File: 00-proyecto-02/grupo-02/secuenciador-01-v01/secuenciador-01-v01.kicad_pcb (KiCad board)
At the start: 2 copper layers, 90 x 50 mm, 18 parts, among them U1 4040, U2 NE555P

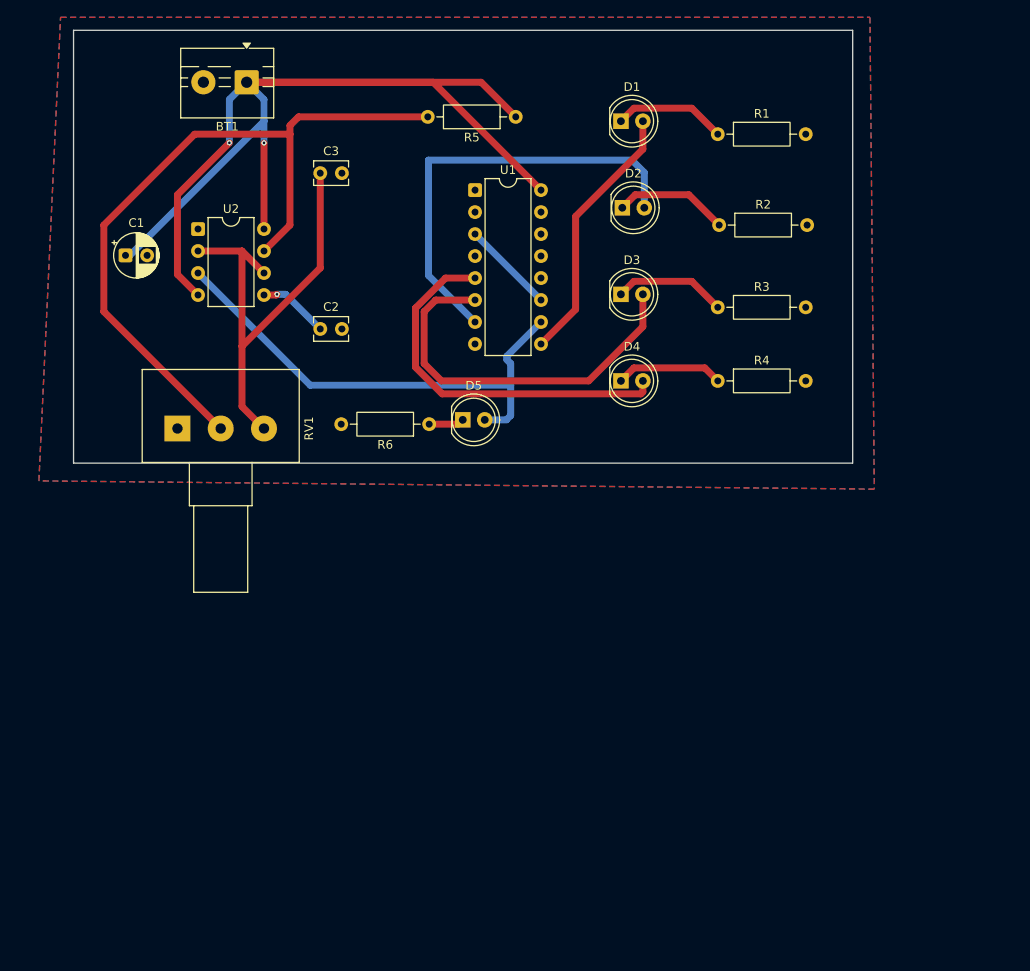
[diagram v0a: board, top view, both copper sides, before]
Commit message: Add files via upload
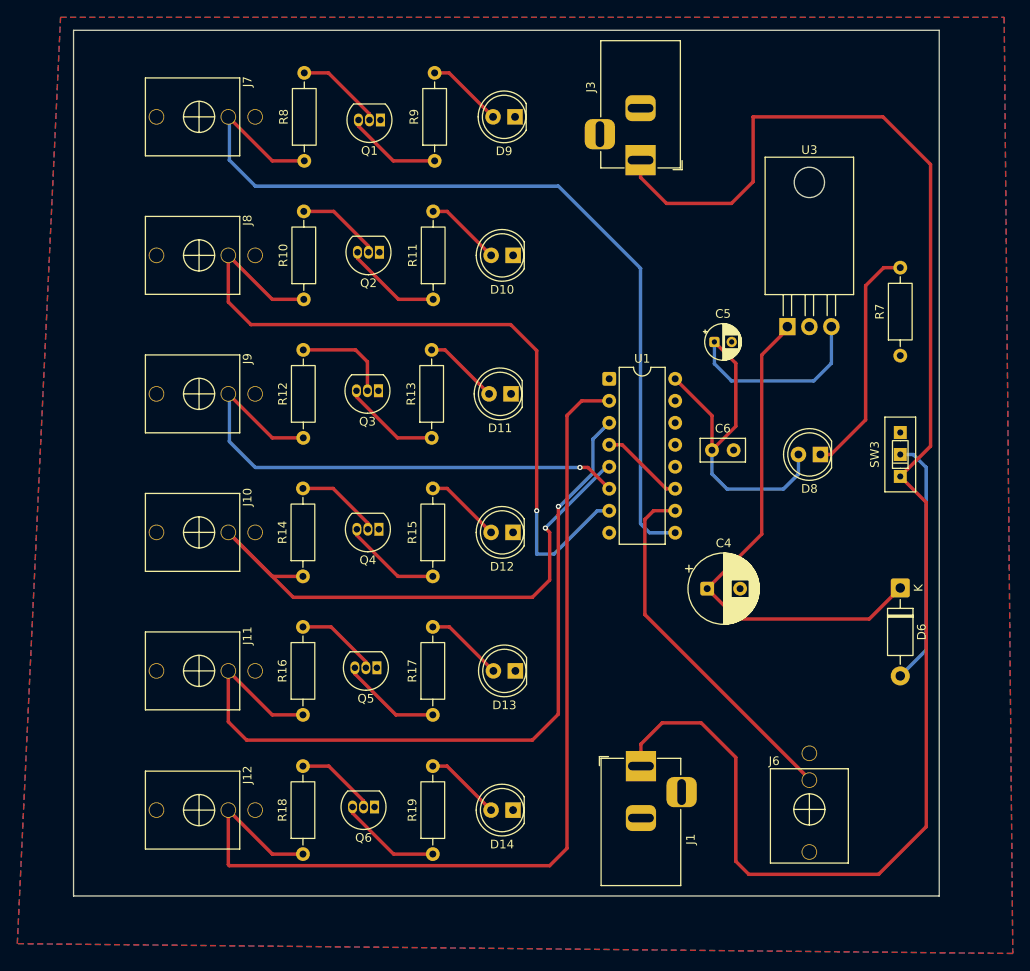
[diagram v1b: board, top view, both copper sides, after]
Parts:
- removed BT1: 9v, TerminalBlock:TerminalBlock_MaiXu_MX126-5.0-02P_1x02_P5.00mm
- removed C1: 100u, Capacitor_THT:CP_Radial_D5.0mm_P2.50mm
- removed C2: 100n, Capacitor_THT:C_Disc_D3.8mm_W2.6mm_P2.50mm
- removed C3: 10n, Capacitor_THT:C_Disc_D3.8mm_W2.6mm_P2.50mm
- removed D1, D2, D3, D4, D5: LED, LED_THT:LED_D5.0mm
- removed R1, R2, R3, R4, R6: 1k, Resistor_THT:R_Axial_DIN0207_L6.3mm_D2.5mm_P10.16mm_Horizontal
- removed R5: 10k, Resistor_THT:R_Axial_DIN0207_L6.3mm_D2.5mm_P10.16mm_Horizontal
- removed RV1: 100k, Potentiometer_THT:Potentiometer_Alps_RK163_Single_Horizontal
- removed U2: NE555P, Package_DIP:DIP-8_W7.62mm
- added C4: 100u, Capacitor_THT:CP_Radial_D8.0mm_P3.80mm, F.Cu at (123.7, 114.5)
- added C5: 10u, Capacitor_THT:CP_Radial_D4.0mm_P2.00mm, F.Cu at (124.5, 86.0)
- added C6: 100n, Capacitor_THT:C_Disc_D5.0mm_W2.5mm_P2.50mm, F.Cu at (124.2, 98.5)
- added D10: LED, LED_THT:LED_D5.0mm, F.Cu at (101.3, 76.0)
- added D11: LED, LED_THT:LED_D5.0mm, F.Cu at (101.0, 92.0)
- added D12: LED, LED_THT:LED_D5.0mm, F.Cu at (101.3, 108.0)
- added D13: LED, LED_THT:LED_D5.0mm, F.Cu at (101.5, 124.0)
- added D14: LED, LED_THT:LED_D5.0mm, F.Cu at (101.3, 140.1)
- added D6: 1N4007, Diode_THT:D_DO-41_SOD81_P10.16mm_Horizontal, F.Cu at (146.0, 114.4)
- added D8: LED, LED_THT:LED_D5.0mm, F.Cu at (136.8, 99.0)
- added D9: LED, LED_THT:LED_D5.0mm, F.Cu at (101.5, 60.0)
- added J1: Barrel_Jack_Switch, Connector_BarrelJack:BarrelJack_Horizontal, F.Cu at (116.0, 135.0)
- added J10: AudioJack2_SwitchT, dis8644:PJ301M-12, F.Cu at (65.0, 108.0)
- added J11: AudioJack2_SwitchT, dis8644:PJ301M-12, F.Cu at (65.0, 124.0)
- added J12: AudioJack2_SwitchT, dis8644:PJ301M-12, F.Cu at (65.0, 140.1)
- added J3: Barrel_Jack_Switch, Connector_BarrelJack:BarrelJack_Horizontal, F.Cu at (116.0, 65.0)
- added J6: AudioJack2_SwitchT, dis8644:PJ301M-12, F.Cu at (135.5, 140.0)
- added J7: AudioJack2_SwitchT, dis8644:PJ301M-12, F.Cu at (65.0, 60.0)
- added J8: AudioJack2_SwitchT, dis8644:PJ301M-12, F.Cu at (65.0, 76.0)
- added J9: AudioJack2_SwitchT, dis8644:PJ301M-12, F.Cu at (65.0, 92.0)
- added Q1: PN2222A, Package_TO_SOT_THT:TO-92_Inline, F.Cu at (86.0, 60.4)
- added Q2: PN2222A, Package_TO_SOT_THT:TO-92_Inline, F.Cu at (85.8, 75.6)
- added Q3: PN2222A, Package_TO_SOT_THT:TO-92_Inline, F.Cu at (85.7, 91.6)
- added Q4: PN2222A, Package_TO_SOT_THT:TO-92_Inline, F.Cu at (85.8, 107.6)
- added Q5: PN2222A, Package_TO_SOT_THT:TO-92_Inline, F.Cu at (85.5, 123.6)
- added Q6: PN2222A, Package_TO_SOT_THT:TO-92_Inline, F.Cu at (85.3, 139.7)
- added R10: 1k, Resistor_THT:R_Axial_DIN0207_L6.3mm_D2.5mm_P10.16mm_Horizontal, F.Cu at (77.1, 81.1)
- added R11: 1k, Resistor_THT:R_Axial_DIN0207_L6.3mm_D2.5mm_P10.16mm_Horizontal, F.Cu at (92.0, 81.1)
- added R12: 1k, Resistor_THT:R_Axial_DIN0207_L6.3mm_D2.5mm_P10.16mm_Horizontal, F.Cu at (77.0, 97.1)
- added R13: 1k, Resistor_THT:R_Axial_DIN0207_L6.3mm_D2.5mm_P10.16mm_Horizontal, F.Cu at (91.9, 97.1)
- added R14: 1k, Resistor_THT:R_Axial_DIN0207_L6.3mm_D2.5mm_P10.16mm_Horizontal, F.Cu at (77.0, 113.1)
- added R15: 1k, Resistor_THT:R_Axial_DIN0207_L6.3mm_D2.5mm_P10.16mm_Horizontal, F.Cu at (92.0, 113.1)
- added R16: 1k, Resistor_THT:R_Axial_DIN0207_L6.3mm_D2.5mm_P10.16mm_Horizontal, F.Cu at (77.0, 129.1)
- added R17: 1k, Resistor_THT:R_Axial_DIN0207_L6.3mm_D2.5mm_P10.16mm_Horizontal, F.Cu at (92.0, 129.1)
- added R18: 1k, Resistor_THT:R_Axial_DIN0207_L6.3mm_D2.5mm_P10.16mm_Horizontal, F.Cu at (77.0, 145.2)
- added R19: 1k, Resistor_THT:R_Axial_DIN0207_L6.3mm_D2.5mm_P10.16mm_Horizontal, F.Cu at (92.0, 145.2)
- added R7: 1k, Resistor_THT:R_Axial_DIN0207_L6.3mm_D2.5mm_P10.16mm_Horizontal, F.Cu at (146.0, 87.6)
- added R8: 1k, Resistor_THT:R_Axial_DIN0207_L6.3mm_D2.5mm_P10.16mm_Horizontal, F.Cu at (77.2, 65.1)
- added R9: 1k, Resistor_THT:R_Axial_DIN0207_L6.3mm_D2.5mm_P10.16mm_Horizontal, F.Cu at (92.2, 65.1)
- added SW3: SW_SPDT, dis8644:spdt_ssd12d00g3, F.Cu at (146.0, 99.0)
- added U3: L7805, Package_TO_SOT_THT:TO-220-3_Horizontal_TabDown, F.Cu at (133.0, 84.2)
- moved U1 26.7 mm to (112.4, 90.3)
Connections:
- U1 pad 11: Net-(U1-Q4) -> Net-(U1-Q6)
- U1 pad 16: VCC -> +5V
- U1 pad 2: unconnected-(U1-Q5-Pad2) -> Net-(U1-Q5)
- U1 pad 4: unconnected-(U1-Q6-Pad4) -> Net-(U1-Q6)
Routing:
- net Net-(SW3-A): track 0.00 -> 179.8 mm
- net VCC: track 141.0 -> 0.00 mm, vias 2 -> 0
- net Net-(U1-Q5): track 0.00 -> 112.6 mm
- net Net-(U2-DISCH): track 87.0 -> 0.00 mm
- net Net-(U1-Q4): track 10.8 -> 93.0 mm, vias 0 -> 1
- net Net-(U1-Q0): track 30.6 -> 102.5 mm
- net +5V: track 0.00 -> 63.5 mm
- net +12V: track 0.00 -> 59.3 mm
- net Net-(U2-THRES): track 54.0 -> 0.00 mm
- net Net-(U1-Q1): track 51.0 -> 88.1 mm, vias 0 -> 1
- net Net-(D6-A): track 0.00 -> 28.9 mm
- net Net-(D8-K): track 0.00 -> 27.2 mm
- net Net-(U1-Q3): track 44.1 -> 68.3 mm, vias 0 -> 1
- net Net-(U1-Q2): track 44.9 -> 62.5 mm, vias 0 -> 1
- net Net-(U1-CLK): track 57.3 -> 41.9 mm
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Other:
- board size 90 x 50 mm -> 100 x 100 mm
